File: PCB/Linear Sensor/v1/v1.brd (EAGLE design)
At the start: 63.5 x 35.8 mm, 43 parts, among them CON1 SPI, IC1 REG1117, Q1 BSP613P, X3 16MHz, X4 MINI-USB-SCHIELD-32005-201

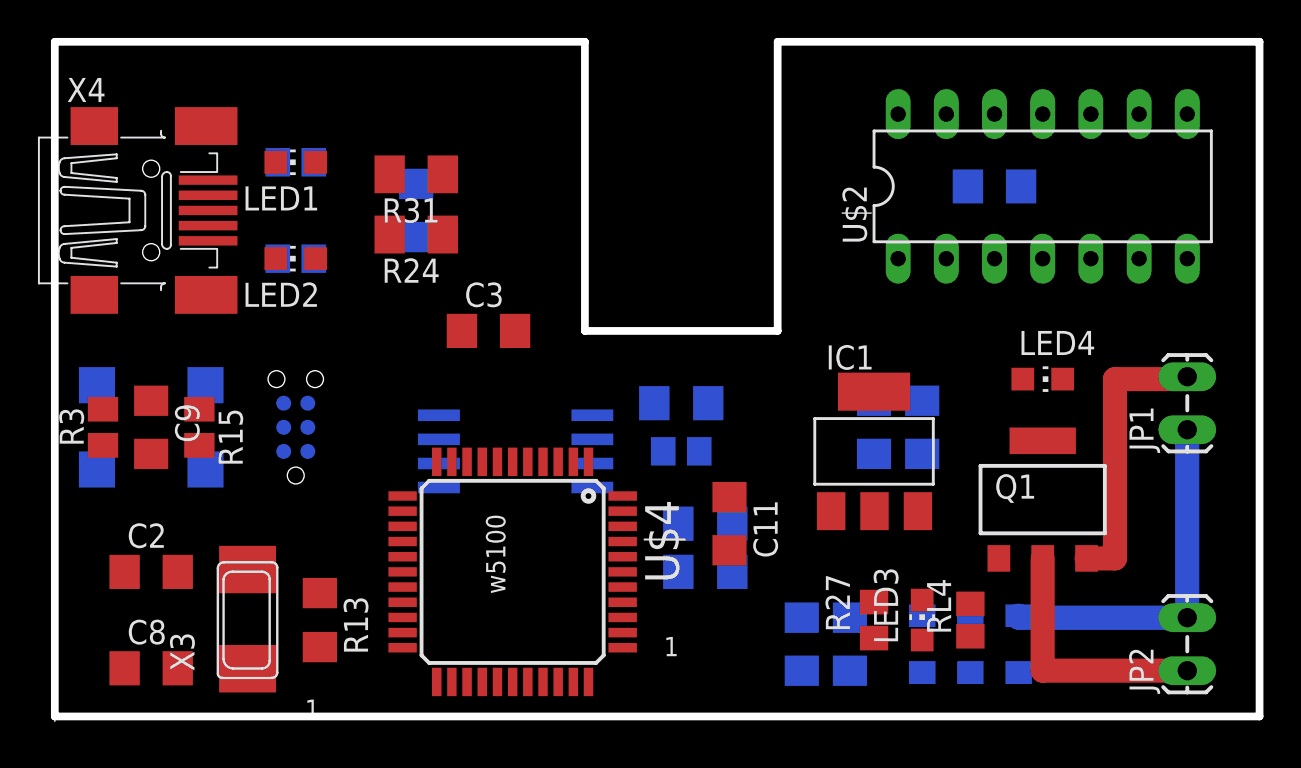
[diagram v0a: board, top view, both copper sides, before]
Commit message: Update cards
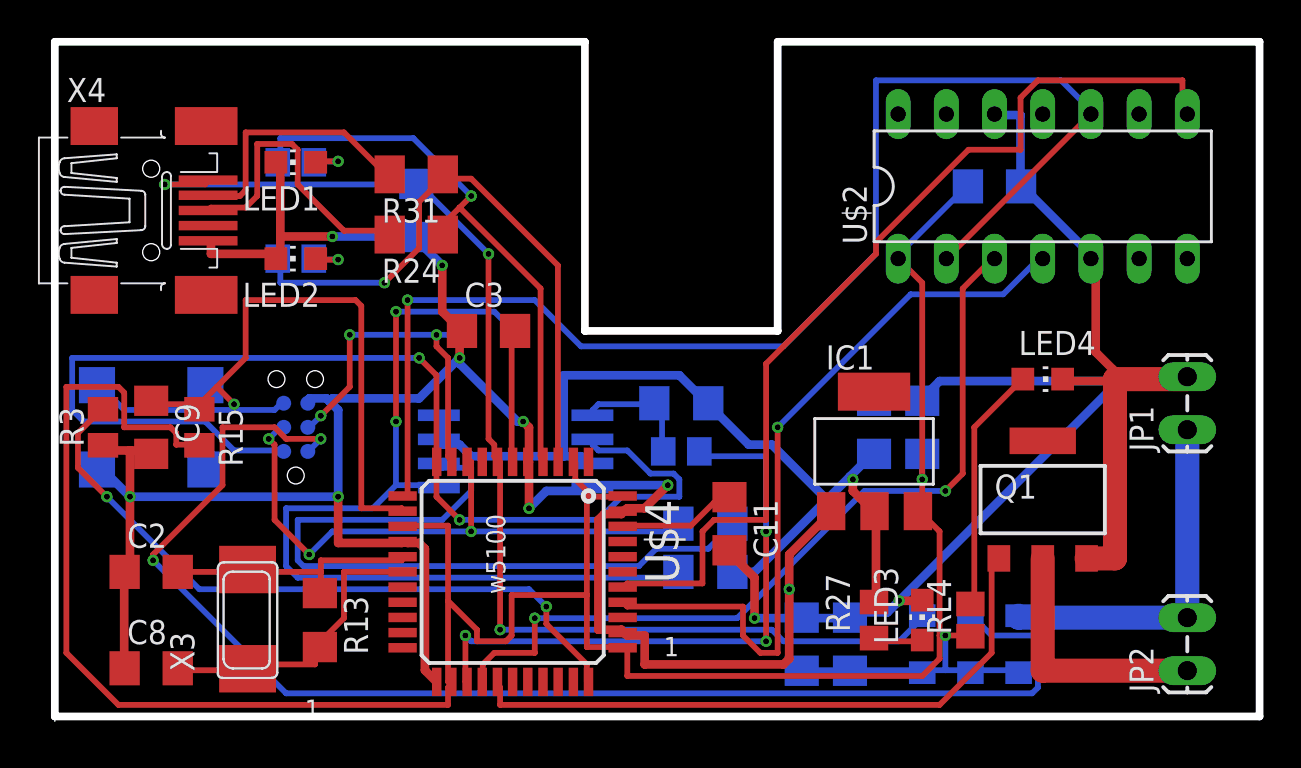
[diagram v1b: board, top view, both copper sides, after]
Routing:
- net GND: track 14.9 -> 213.8 mm, vias 0 -> 11
- net +5V/1: track 0.00 -> 144.8 mm, vias 0 -> 2
- net ISP+5V: track 0.00 -> 71.3 mm, vias 0 -> 2
- net D11*: track 0.00 -> 70.4 mm, vias 0 -> 1
- net VUSB: track 0.00 -> 64.2 mm, vias 0 -> 3
- net MISO: track 0.00 -> 61.1 mm, vias 0 -> 2
- net A2: track 0.00 -> 50.8 mm
- net FMOSI: track 0.00 -> 48.6 mm, vias 0 -> 2
- net 3.3V: track 0.00 -> 48.4 mm, vias 0 -> 1
- net D12*: track 0.00 -> 43.5 mm, vias 0 -> 2
- net RESET: track 0.00 -> 41.0 mm, vias 0 -> 1
- net A1: track 0.00 -> 39.7 mm, vias 0 -> 1
- net N$23: track 0.00 -> 38.9 mm
- net HWB: track 0.00 -> 36.3 mm, vias 0 -> 2
- net D6*: track 0.00 -> 33.4 mm
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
